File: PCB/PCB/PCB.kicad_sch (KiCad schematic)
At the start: 8 parts, among them Q1 2N3905, Q2 2N3905, U1 ESP32-S3, U2 CP2104

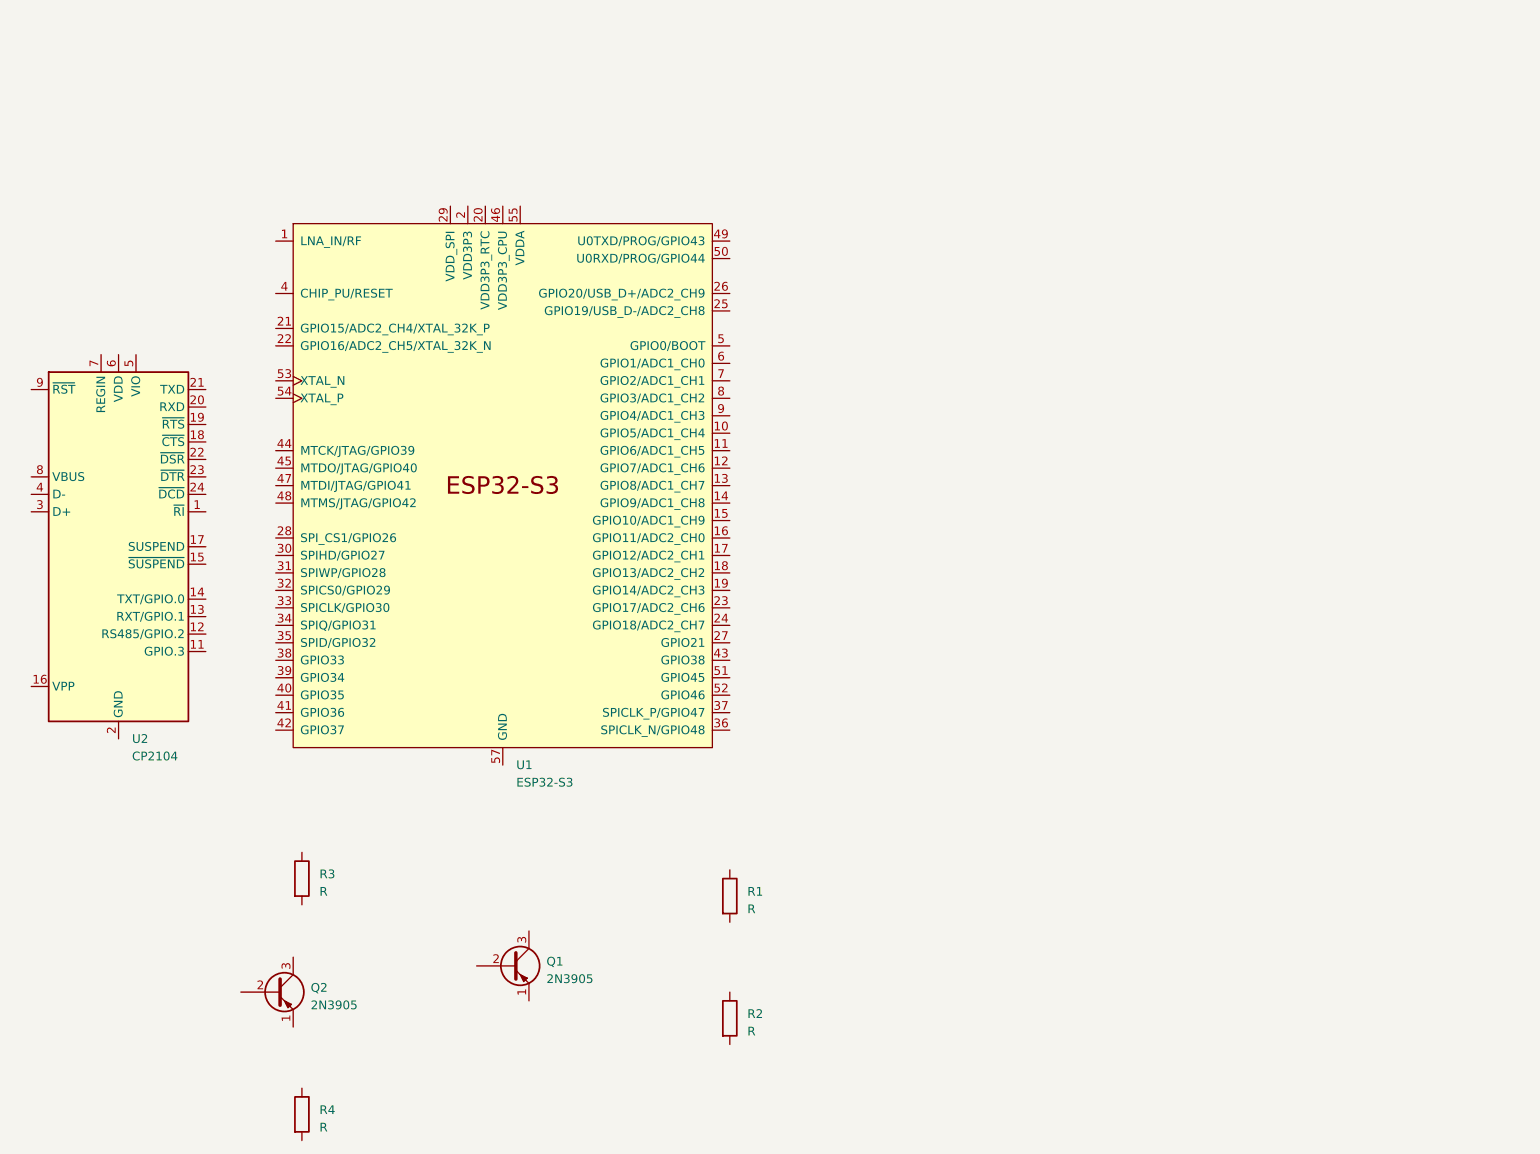
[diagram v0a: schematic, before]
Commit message: first PCB draft
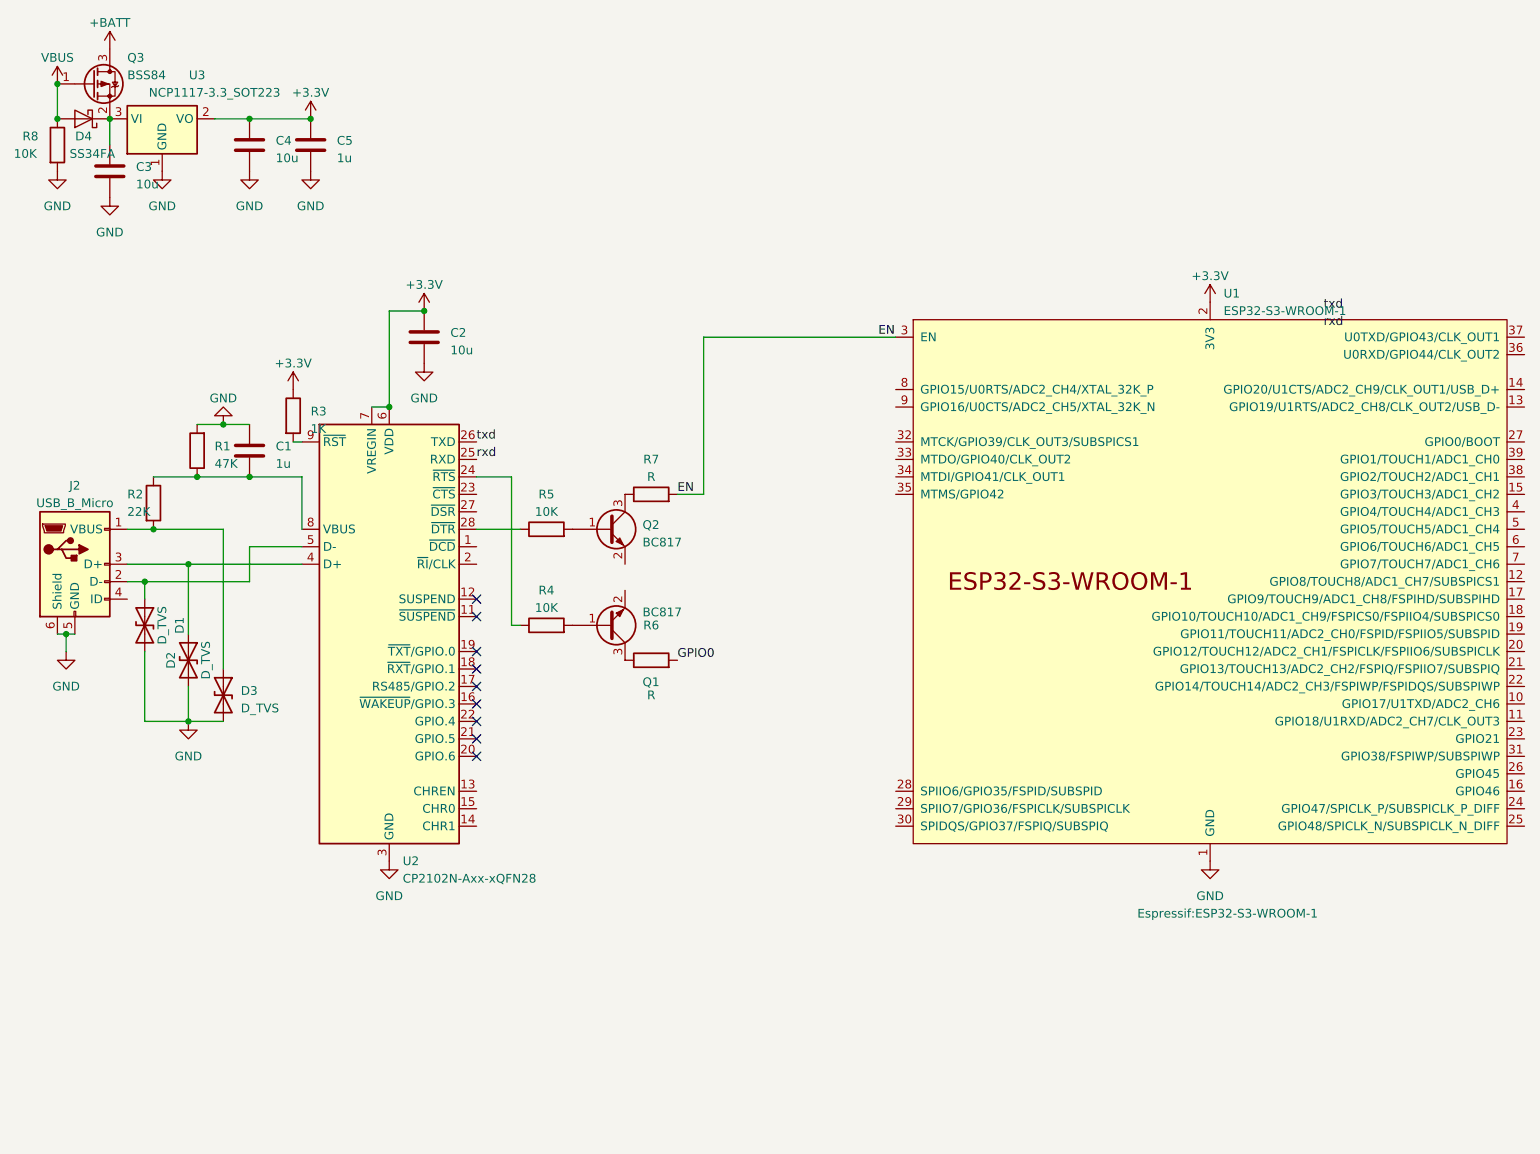
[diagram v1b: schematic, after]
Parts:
- removed Q1, Q2: 2N3905, Package_TO_SOT_THT:TO-92_Inline, symbol Transistor_BJT:2N3905
- removed U1: ESP32-S3, Package_DFN_QFN:QFN-56-1EP_7x7mm_P0.4mm_EP5.6x5.6mm, symbol Espressif:ESP32-S3
- removed U2: CP2104, Package_DFN_QFN:QFN-24-1EP_4x4mm_P0.5mm_EP2.6x2.6mm, symbol Interface_USB:CP2104
- added C1, C5: 1u, symbol Device:C
- added C2, C3, C4: 10u, symbol Device:C
- added D1, D2, D3: D_TVS, Diode_SMD:D_0603_1608Metric, symbol Device:D_TVS
- added D4: SS34FA, Diode_SMD:D_SOD-123F, symbol Diode:MBR1020VL
- added J2: USB_B_Micro, Connector_USB:USB_Micro-B_Molex-105017-0001, symbol Connector:USB_B_Micro
- added Q1, Q2: BC817, Package_TO_SOT_SMD:SOT-23, symbol Transistor_BJT:BC817
- added Q3: BSS84, Package_TO_SOT_SMD:SOT-23, symbol Transistor_FET:BSS84
- added R5, R8: 10K, symbol Device:R
- added R6, R7: R, symbol Device:R
- added U1: ESP32-S3-WROOM-1, Espressif:ESP32-S3-WROOM-1, symbol Espressif:ESP32-S3-WROOM-1
- added U2: CP2102N-Axx-xQFN28, Package_DFN_QFN:QFN-28-1EP_5x5mm_P0.5mm_EP3.35x3.35mm, symbol Interface_USB:CP2102N-Axx-xQFN28
- added U3: NCP1117-3.3_SOT223, Package_TO_SOT_SMD:SOT-223-3_TabPin2, symbol Regulator_Linear:NCP1117-3.3_SOT223
- R1: value R -> 47K
- R2: value R -> 22K
- R3: value R -> 1K
- R4: value R -> 10K
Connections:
- net at R2.1: now also R1.1, C1.2, U2.8 (VBUS)
- net at R2.2: now also D3.1 (A1), J2.1 (VBUS)
- net at R4.1: now also U2.24 (~{RTS})
- net at R4.2: now also Q1.1 (B)
- net +3.3V: now reaches R3.1
- net +3.3V: now also C2.1, C4.1, C5.1, U1.2 (3V3), U2.6 (VDD), U2.7 (VREGIN), U3.2 (VO)
- net at R3.2: now also U2.9 (~{RST})
- net GND: now reaches R1.2
- net GND: now also C1.1, C2.2, C3.2, C4.2, C5.2, D1.2 (A2), D2.2 (A2), D3.2 (A2), J2.5 (GND), J2.6 (Shield), R8.2, U1.1 (GND), U1.40 (GND), U1.41 (GND), U2.29 (GND), U2.3 (GND), U3.1 (GND)
- new net: Q1.3 (C), R6.1
- new net: D1.1 (A1), J2.2 (D-), U2.5 (D-)
- new net: D2.1 (A1), J2.3 (D+), U2.4 (D+)
- new net: Q2.1 (B), R5.2
- new net: Q2.3 (C), R7.1
- new net: R5.1, U2.28 (~{DTR})
- new net: C3.1, D4.1 (K), Q3.2 (S), U3.3 (VI)
- new net +BATT: Q3.3 (D)
- new net EN: R7.2, U1.3 (EN)
- new net GPIO0: R6.2
- new net VBUS: D4.2 (A), Q3.1 (G), R8.1
- new net rxd: U2.25 (RXD)
- new net txd: U2.26 (TXD)
- no-connect marks 0 -> 9
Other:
- moved on the sheet: R1, R2, R3, R4
